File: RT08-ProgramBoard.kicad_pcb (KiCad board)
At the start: 2 copper layers, 309 parts, among them J1 PWR/Addr, J2 Instruction, J3 Data, J4 Instruction, J5 Data

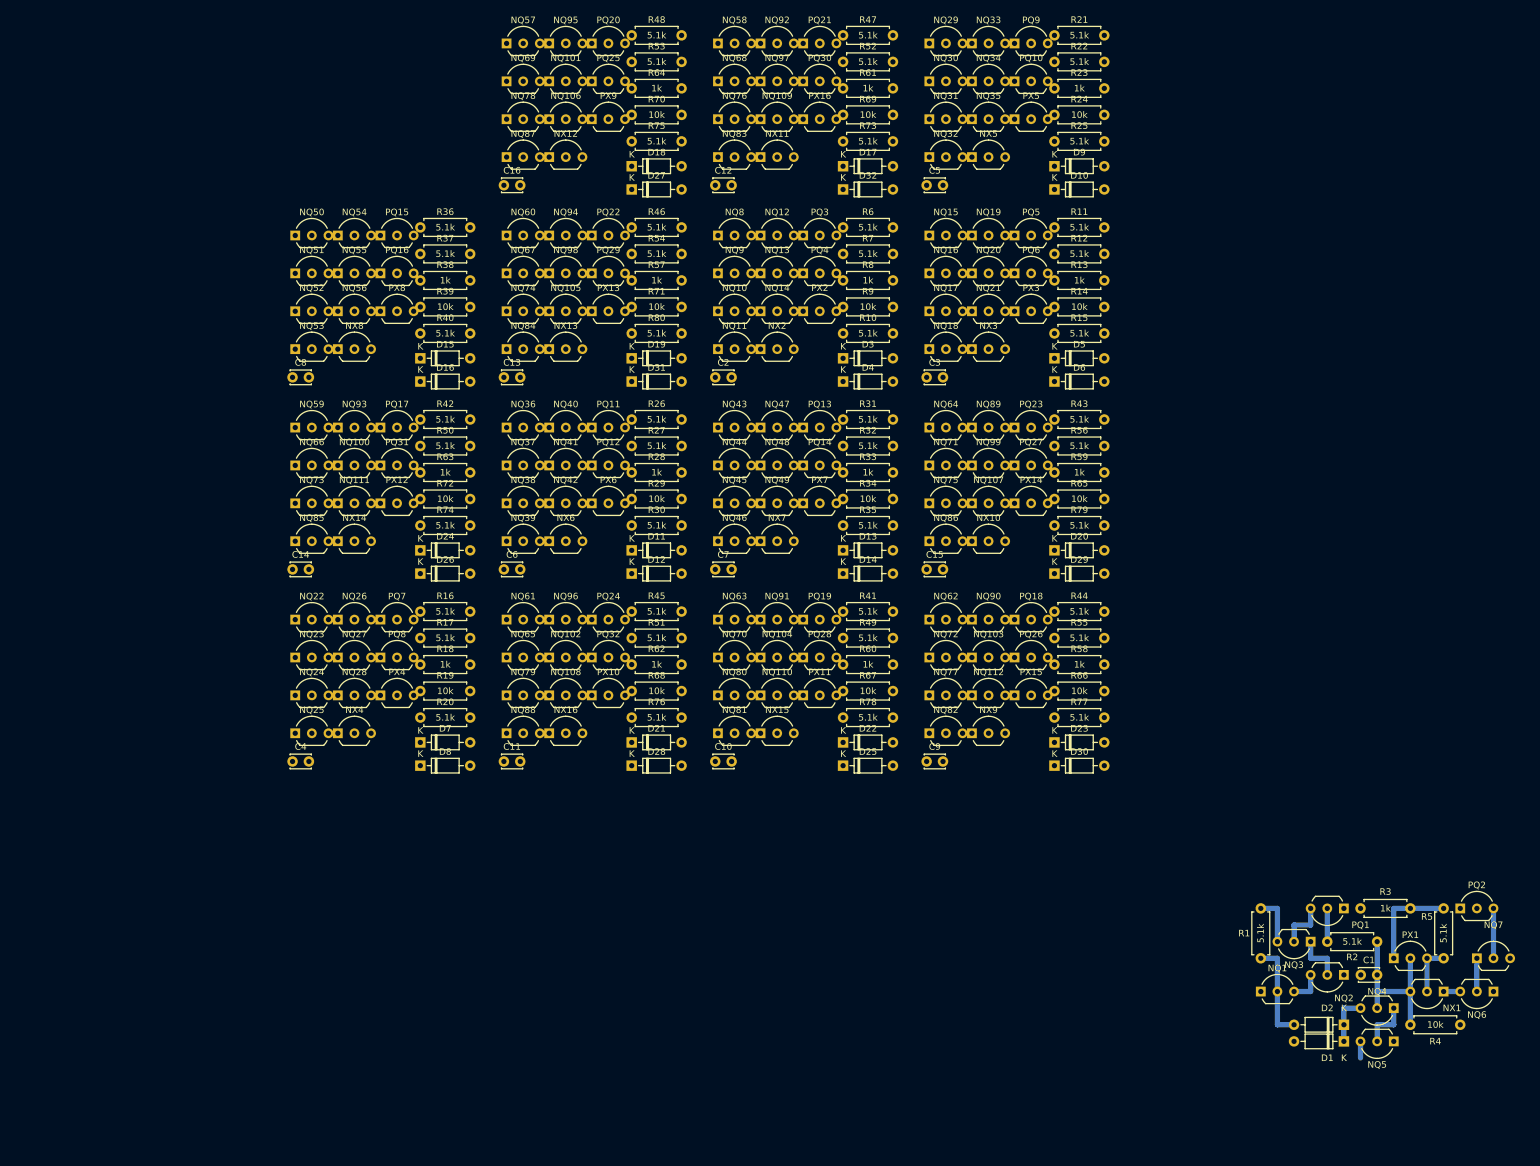
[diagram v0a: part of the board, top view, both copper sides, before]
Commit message: Assembled 4 cells, fp copied
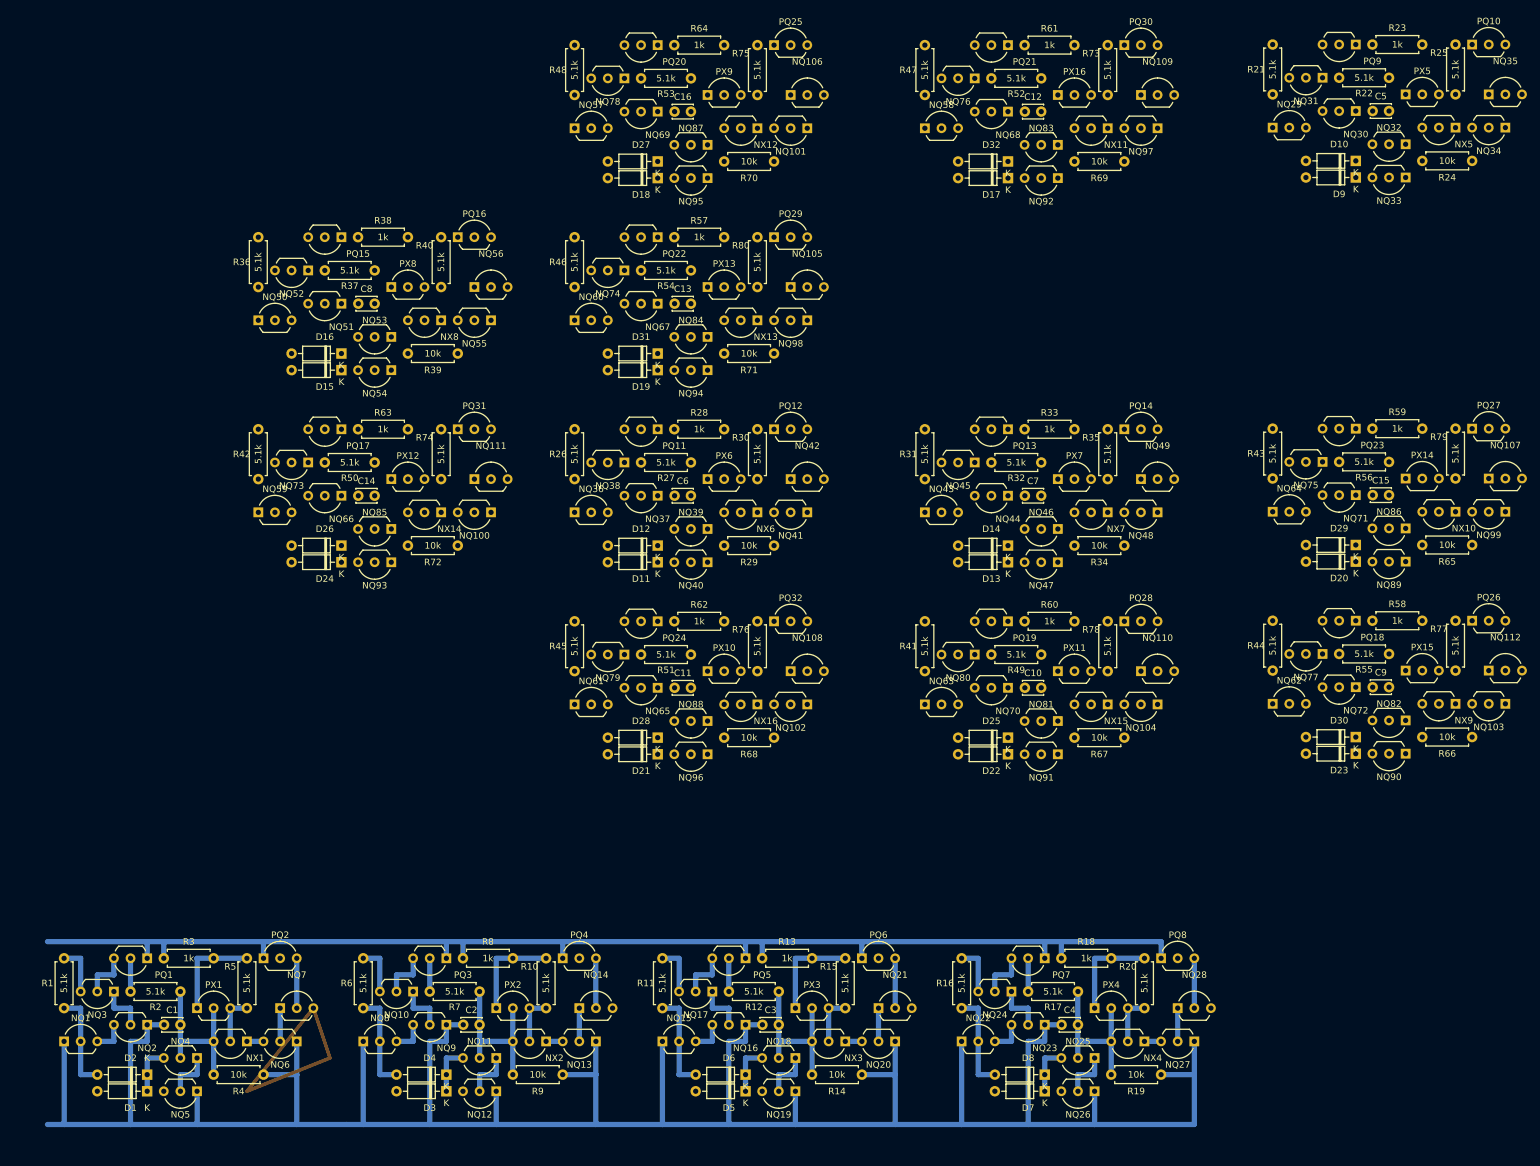
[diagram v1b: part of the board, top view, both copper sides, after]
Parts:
- moved NQ1 183.0 mm to (30.5, 172.7)
- moved R1 183.0 mm to (30.5, 160.0)
- moved C1 183.0 mm to (45.8, 170.2)
- moved D1 183.0 mm to (43.2, 180.3)
- moved D2 183.0 mm to (43.2, 177.8)
- moved NQ2 183.0 mm to (43.2, 170.2)
- moved NQ3 183.0 mm to (38.1, 165.1)
- moved NQ4 183.0 mm to (50.8, 175.3)
- moved NQ5 183.0 mm to (50.8, 180.3)
- moved NQ6 183.0 mm to (66.0, 172.7)
- moved NQ7 183.0 mm to (63.5, 167.6)
- moved NX1 183.0 mm to (58.4, 172.7)
- moved PQ1 183.0 mm to (43.2, 160.0)
- moved PQ2 183.0 mm to (61.0, 160.0)
- moved PX1 183.0 mm to (50.8, 167.6)
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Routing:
- net GND: track 0.00 -> 398.9 mm
- net +5V: track 0.00 -> 200.7 mm
- net Net-(NQ25-C): track 0.00 -> 25.4 mm
- net Net-(NQ18-C): track 0.00 -> 25.4 mm
- net Net-(NQ11-C): track 0.00 -> 25.4 mm
- net /WEn: track 10.2 -> 30.5 mm
- net Net-(D8-A): track 0.00 -> 15.2 mm
- net Net-(D6-A): track 0.00 -> 15.2 mm
- net Net-(D4-A): track 0.00 -> 15.2 mm
- net Net-(PX4-E): track 0.00 -> 15.2 mm
- net Net-(PX3-E): track 0.00 -> 15.2 mm
- net Net-(PX2-E): track 0.00 -> 15.2 mm
- net Net-(NX4-C): track 0.00 -> 7.62 mm
- net Net-(NX3-C): track 0.00 -> 7.62 mm
- net Net-(NQ25-E): track 0.00 -> 7.62 mm
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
